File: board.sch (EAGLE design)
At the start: 13 parts

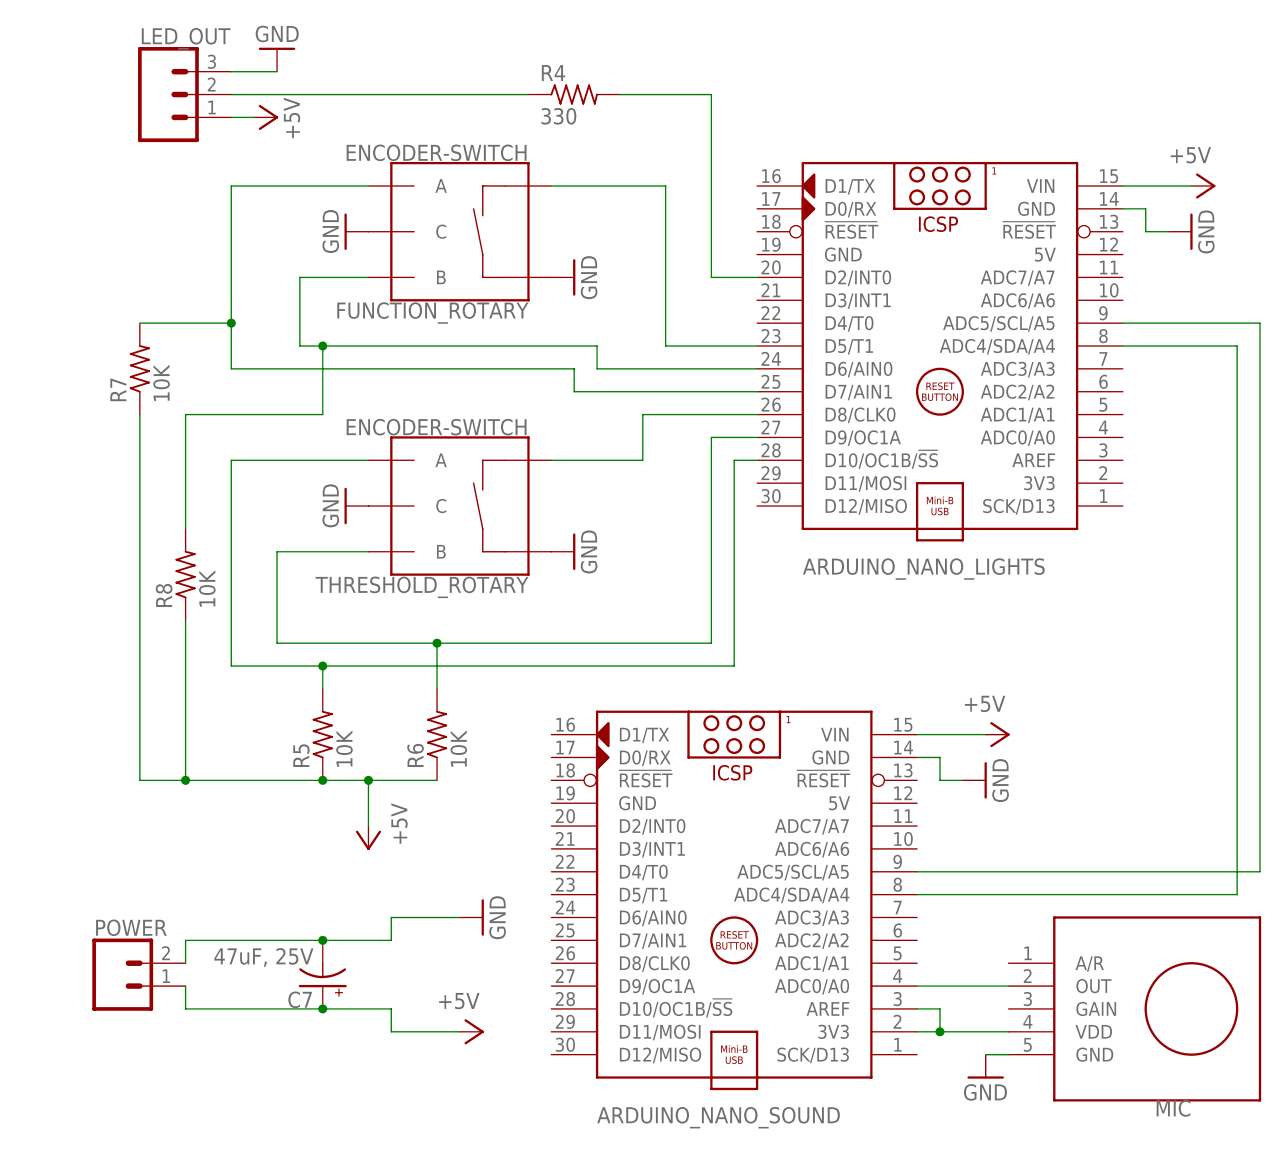
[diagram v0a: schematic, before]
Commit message: Updating schematic
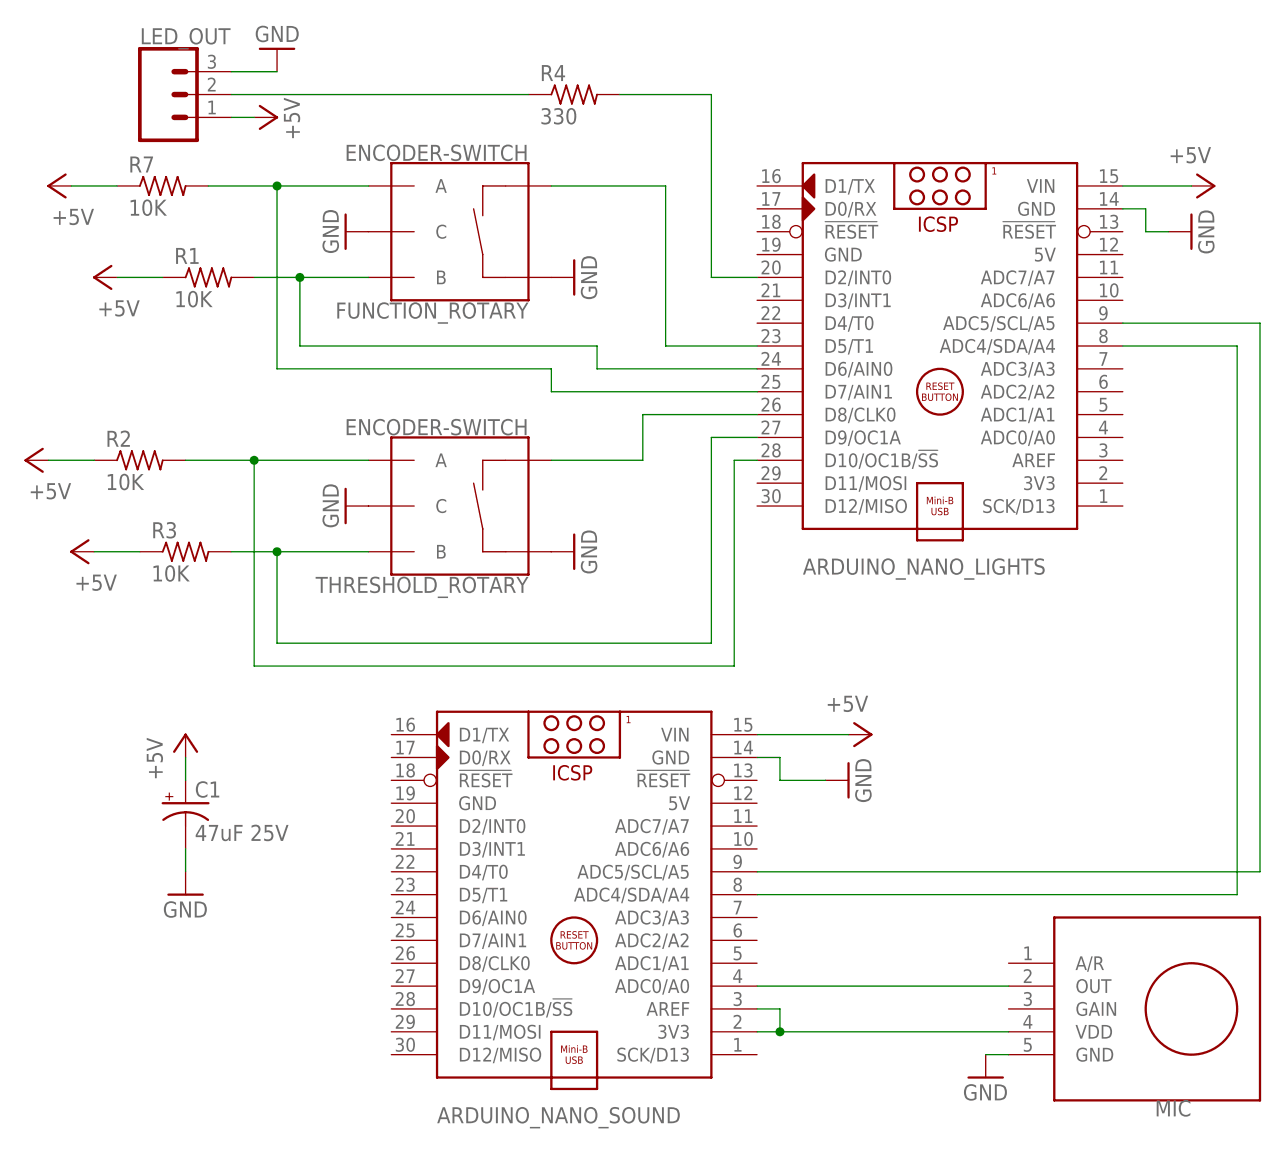
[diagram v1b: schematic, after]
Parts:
- removed C7: 47uF, 25V, rcl:CPOL-USE2-5
- removed POWER: (no value), SparkFun-Connectors:CONN_02
- removed R5, R6, R8: 10K, adafruit:R-US_0207/7
- added C1: 47uF 25V, adafruit:CPOL-USE2-5
- added R1, R2, R3: 10K, adafruit:R-US_0207/7
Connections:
- removed net N$14: ARDUINO_NANO_LIGHTS.D6/AIN0, FUNCTION_ROTARY.B, R8.2
- new net N$4: ARDUINO_NANO_LIGHTS.D6/AIN0, FUNCTION_ROTARY.B, R1.2
- net +5V: now also C1.+, R1.1, R2.1, R3.1; no longer C7.+, POWER.1, R5.1, R6.1, R8.1
- net GND: now also C1.-; no longer C7.-, POWER.2
- net N$15: now also R2.2; no longer R5.2
- net N$2: now also R3.2; no longer R6.2
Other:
- moved on the sheet: ARDUINO_NANO_SOUND, R7

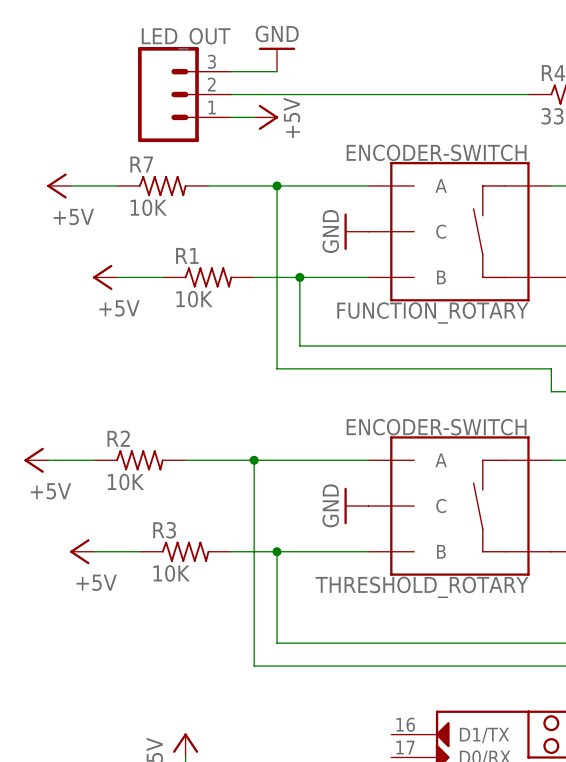
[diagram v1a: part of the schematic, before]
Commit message: V2, applying learnings from V1
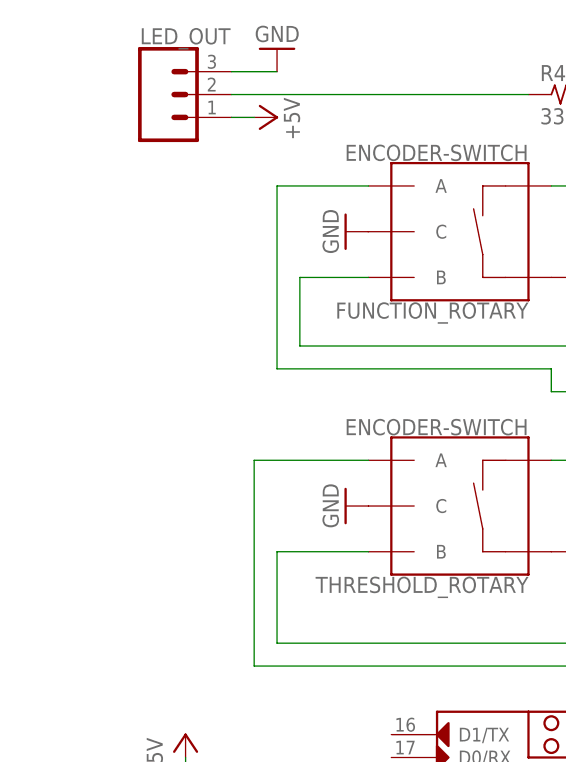
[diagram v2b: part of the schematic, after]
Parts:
- removed R1, R2, R3, R7: 10K, adafruit:R-US_0207/7
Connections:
- net +5V: no longer R1.1, R2.1, R3.1, R7.1
- net N$13: no longer R7.2
- net N$15: no longer R2.2
- net N$2: no longer R3.2
- net N$4: no longer R1.2
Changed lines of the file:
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@@
 <part name="GND14" library="supply1" deviceset="GND" device=""/>
 <part name="GND15" library="supply1" deviceset="GND" device=""/>
-<part name="R7" library="adafruit" library_urn="urn:adsk.eagle:library:420" deviceset="R-US_" device="0207/7" package3d_urn="urn:adsk.eagle:package:6240602/1" value="10K"/>
 <part name="P+4" library="supply1" library_urn="urn:adsk.eagle:library:371" deviceset="+5V" device=""/>
 <part name="P+5" library="supply1" library_urn="urn:adsk.eagle:library:371" deviceset="+5V" device=""/>
@@
 <part name="MIC" library="toepferg" deviceset="ADAFRUIT_ELECTRET_MIC_MAX9817" device=""/>
 <part name="GND16" library="supply1" deviceset="GND" device=""/>
-<part name="P+1" library="supply1" library_urn="urn:adsk.eagle:library:371" deviceset="+5V" device=""/>
-<part name="R1" library="adafruit" library_urn="urn:adsk.eagle:library:420" deviceset="R-US_" device="0207/7" package3d_urn="urn:adsk.eagle:package:6240602/1" value="10K"/>
-<part name="P+7" library="supply1" library_urn="urn:adsk.eagle:library:371" deviceset="+5V" device=""/>
-<part name="R2" library="adafruit" library_urn="urn:adsk.eagle:library:420" deviceset="R-US_" device="0207/7" package3d_urn="urn:adsk.eagle:package:6240602/1" value="10K"/>
-<part name="P+8" library="supply1" library_urn="urn:adsk.eagle:library:371" deviceset="+5V" device=""/>
-<part name="R3" library="adafruit" library_urn="urn:adsk.eagle:library:420" deviceset="R-US_" device="0207/7" package3d_urn="urn:adsk.eagle:package:6240602/1" value="10K"/>
-<part name="P+9" library="supply1" library_urn="urn:adsk.eagle:library:371" deviceset="+5V" device=""/>
 <part name="P+2" library="supply1" library_urn="urn:adsk.eagle:library:371" deviceset="+5V" device=""/>
 <part name="GND2" library="supply1" deviceset="GND" device=""/>
@@
 <attribute name="VALUE" x="-15.24" y="154.94" size="1.778" layer="96" rot="R180"/>
 </instance>
-<instance part="R7" gate="G$1" x="-30.48" y="137.16" smashed="yes">
-<attribute name="NAME" x="-34.29" y="138.6586" size="1.778" layer="95"/>
-<attribute name="VALUE" x="-34.29" y="133.858" size="1.778" layer="96"/>
-</instance>
 <instance part="P+4" gate="1" x="-17.78" y="144.78" smashed="yes" rot="R270">
 <attribute name="VALUE" x="-15.24" y="142.24" size="1.778" layer="96" rot="R90"/>
@@
 <instance part="GND16" gate="1" x="60.96" y="38.1" smashed="yes">
 <attribute name="VALUE" x="58.42" y="35.56" size="1.778" layer="96"/>
-</instance>
-<instance part="P+1" gate="1" x="-43.18" y="137.16" smashed="yes" rot="R90">
-<attribute name="VALUE" x="-38.1" y="134.62" size="1.778" layer="96" rot="R180"/>
-</instance>
-<instance part="R1" gate="G$1" x="-25.4" y="127" smashed="yes">
-<attribute name="NAME" x="-29.21" y="128.4986" size="1.778" layer="95"/>
-<attribute name="VALUE" x="-29.21" y="123.698" size="1.778" layer="96"/>
-</instance>
-<instance part="P+7" gate="1" x="-38.1" y="127" smashed="yes" rot="R90">
-<attribute name="VALUE" x="-33.02" y="124.46" size="1.778" layer="96" rot="R180"/>
-</instance>
-<instance part="R2" gate="G$1" x="-33.02" y="106.68" smashed="yes">
-<attribute name="NAME" x="-36.83" y="108.1786" size="1.778" layer="95"/>
-<attribute name="VALUE" x="-36.83" y="103.378" size="1.778" layer="96"/>
-</instance>
-<instance part="P+8" gate="1" x="-45.72" y="106.68" smashed="yes" rot="R90">
-<attribute name="VALUE" x="-40.64" y="104.14" size="1.778" layer="96" rot="R180"/>
-</instance>
-<instance part="R3" gate="G$1" x="-27.94" y="96.52" smashed="yes">
-<attribute name="NAME" x="-31.75" y="98.0186" size="1.778" layer="95"/>
-<attribute name="VALUE" x="-31.75" y="93.218" size="1.778" layer="96"/>
-</instance>
-<instance part="P+9" gate="1" x="-40.64" y="96.52" smashed="yes" rot="R90">
-<attribute name="VALUE" x="-35.56" y="93.98" size="1.778" layer="96" rot="R180"/>
 </instance>
 <instance part="P+2" gate="1" x="-27.94" y="76.2" smashed="yes">
@@
 <wire x1="-17.78" y1="96.52" x2="-7.62" y2="96.52" width="0.1524" layer="91"/>
 <wire x1="-17.78" y1="86.36" x2="-17.78" y2="96.52" width="0.1524" layer="91"/>
-<pinref part="R3" gate="G$1" pin="2"/>
-<wire x1="-17.78" y1="96.52" x2="-22.86" y2="96.52" width="0.1524" layer="91"/>
-<junction x="-17.78" y="96.52"/>
 </segment>
 </net>
@@
 <wire x1="12.7" y1="114.3" x2="35.56" y2="114.3" width="0.1524" layer="91"/>
 <wire x1="-17.78" y1="137.16" x2="-17.78" y2="116.84" width="0.1524" layer="91"/>
-<pinref part="R7" gate="G$1" pin="2"/>
-<wire x1="-17.78" y1="137.16" x2="-25.4" y2="137.16" width="0.1524" layer="91"/>
-<junction x="-17.78" y="137.16"/>
 </segment>
 </net>
@@
 <wire x1="33.02" y1="83.82" x2="-20.32" y2="83.82" width="0.1524" layer="91"/>
 <wire x1="-20.32" y1="83.82" x2="-20.32" y2="106.68" width="0.1524" layer="91"/>
-<pinref part="R2" gate="G$1" pin="2"/>
-<wire x1="-20.32" y1="106.68" x2="-27.94" y2="106.68" width="0.1524" layer="91"/>
-<junction x="-20.32" y="106.68"/>
 </segment>
 </net>
@@
 <pinref part="P+4" gate="1" pin="+5V"/>
 <wire x1="-22.86" y1="144.78" x2="-20.32" y2="144.78" width="0.1524" layer="91"/>
-</segment>
-<segment>
-<pinref part="R7" gate="G$1" pin="1"/>
-<pinref part="P+1" gate="1" pin="+5V"/>
-<wire x1="-35.56" y1="137.16" x2="-40.64" y2="137.16" width="0.1524" layer="91"/>
-</segment>
-<segment>
-<pinref part="R1" gate="G$1" pin="1"/>
-<pinref part="P+7" gate="1" pin="+5V"/>
-<wire x1="-30.48" y1="127" x2="-35.56" y2="127" width="0.1524" layer="91"/>
-</segment>
-<segment>
-<pinref part="R2" gate="G$1" pin="1"/>
-<pinref part="P+8" gate="1" pin="+5V"/>
-<wire x1="-38.1" y1="106.68" x2="-43.18" y2="106.68" width="0.1524" layer="91"/>
-</segment>
-<segment>
-<pinref part="R3" gate="G$1" pin="1"/>
-<pinref part="P+9" gate="1" pin="+5V"/>
-<wire x1="-33.02" y1="96.52" x2="-38.1" y2="96.52" width="0.1524" layer="91"/>
 </segment>
 <segment>
@@
 <net name="N$4" class="0">
 <segment>
-<pinref part="R1" gate="G$1" pin="2"/>
-<wire x1="-15.24" y1="127" x2="-20.32" y2="127" width="0.1524" layer="91"/>
 <pinref part="FUNCTION_ROTARY" gate="G$1" pin="B"/>
 <wire x1="-15.24" y1="127" x2="-7.62" y2="127" width="0.1524" layer="91"/>
@@
 <wire x1="17.78" y1="116.84" x2="35.56" y2="116.84" width="0.1524" layer="91"/>
 <wire x1="-15.24" y1="127" x2="-15.24" y2="119.38" width="0.1524" layer="91"/>
-<junction x="-15.24" y="127"/>
 </segment>
 </net>
@@
 </sheet>
 </sheets>
+<errors>
+</errors>
 </schematic>
 </drawing>
